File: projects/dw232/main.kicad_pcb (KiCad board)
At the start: 4 copper layers, 100 x 30 mm, 33 parts, among them P101 CONN_01X11, Q501 MMBT3904, Q502 MMBT3904, U501 LM741, U502 LM741, U503 2DW232

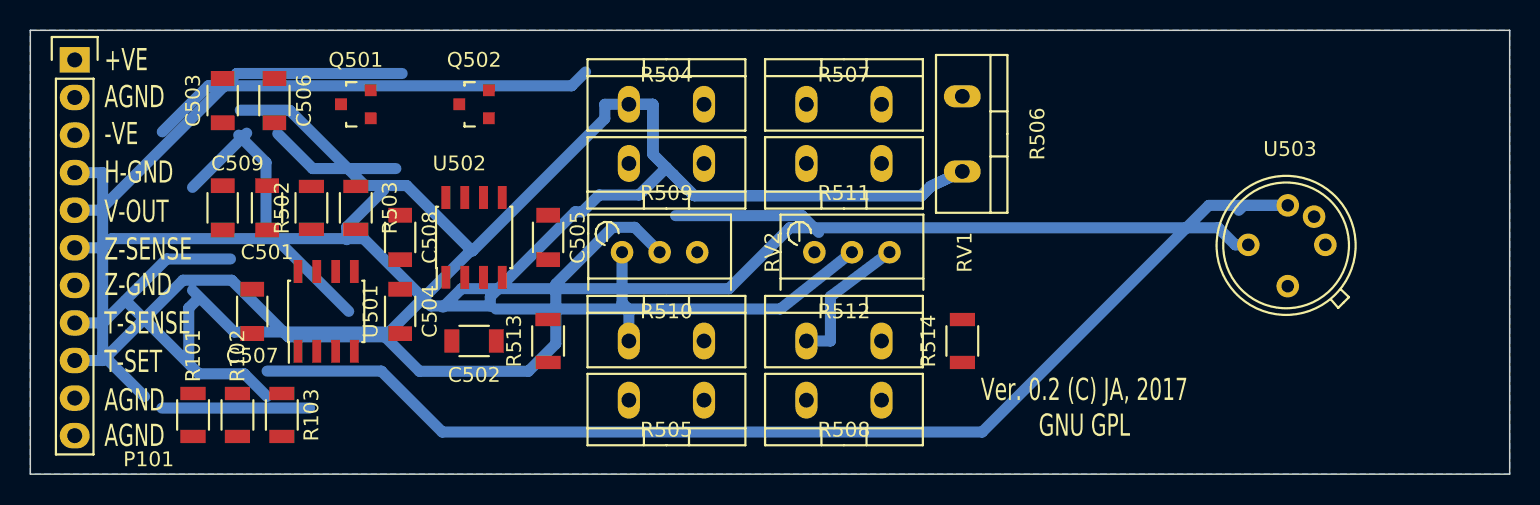
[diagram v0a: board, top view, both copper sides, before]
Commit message: ok, routed and reasonable
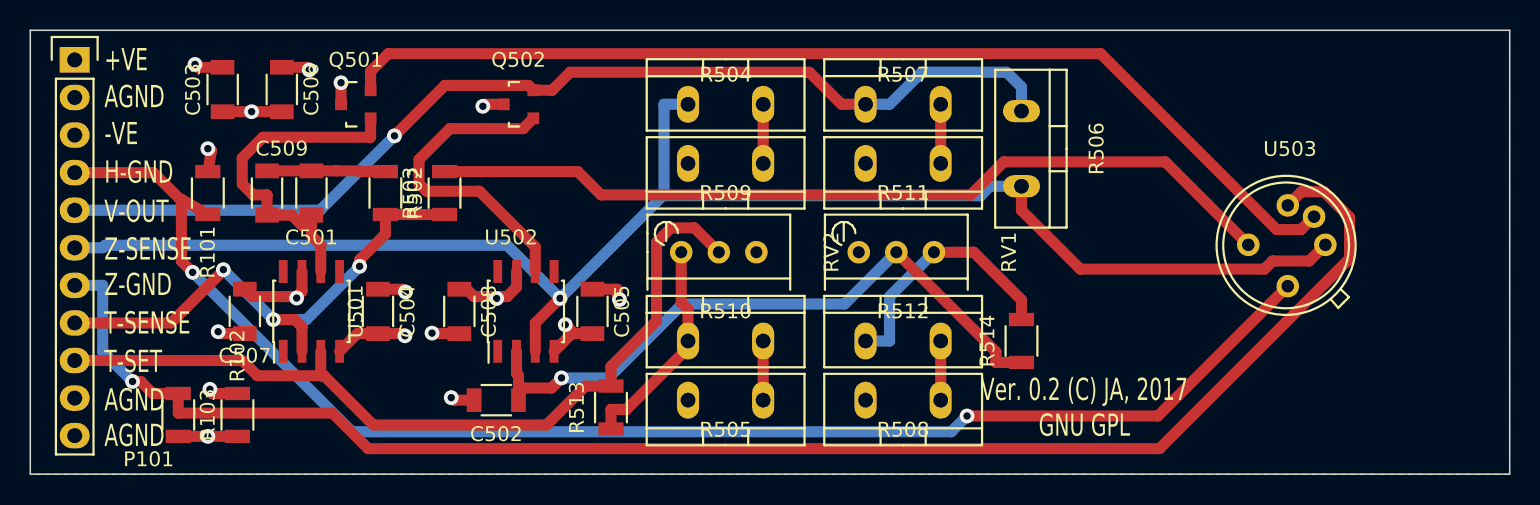
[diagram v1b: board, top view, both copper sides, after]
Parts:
- moved R101 15.0 mm to (51.0, 40.0), turned to 90 degrees
- moved R103 7.00 mm to (49.0, 55.0)
- moved C508 6.40 mm to (68.0, 48.0)
- moved R513 6.19 mm to (78.2, 54.5)
- moved U502 6.10 mm to (72.5, 48.0)
- moved R503 6.08 mm to (67.0, 40.0), turned to 90 degrees
- moved C505 5.83 mm to (77.0, 48.0)
- moved R502 5.10 mm to (63.0, 40.0), turned to 90 degrees
- moved C502 4.27 mm to (70.5, 54.0)
- moved R506 4.12 mm to (106.0, 37.0)
- moved R504 4.00 mm to (86.0, 34.0)
- moved R505 4.00 mm to (86.0, 54.0)
- moved R507 4.00 mm to (98.0, 34.0)
- moved R508 4.00 mm to (98.0, 54.0)
- moved R509 4.00 mm to (86.0, 38.0)
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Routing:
- net (no net): track 143.1 -> 0.00 mm
- net H-GND: track 18.2 -> 97.8 mm, vias 0 -> 2
- net Net-(Q501-Pad2): track 0.00 -> 70.8 mm
- net Z-SENSE: track 158.7 -> 105.3 mm, vias 0 -> 1
- net V-OUT: track 26.1 -> 72.0 mm, vias 0 -> 1
- net Z-SENSE-GND: track 80.5 -> 107.5 mm, vias 0 -> 1
- net T-SENSE: track 12.3 -> 35.7 mm, vias 0 -> 3
- net Net-(C501-Pad2): track 0.00 -> 23.0 mm
- net Net-(Q502-Pad1): track 0.00 -> 21.8 mm
- net AGND: track 0.00 -> 19.4 mm, vias 0 -> 8
- net Net-(C502-Pad1): track 25.4 -> 44.7 mm, vias 0 -> 1
- net +VE: track 0.00 -> 16.5 mm, vias 0 -> 5
- net -VE: track 0.00 -> 12.9 mm, vias 0 -> 4
- net Net-(R509-Pad2): track 0.00 -> 8.87 mm
- net Net-(R510-Pad1): track 6.19 -> 14.9 mm
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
